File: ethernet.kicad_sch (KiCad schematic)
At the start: 22 parts, among them J2 L834-1G1T-S7, Q2 PMOS_Substrate, U2 LAN8830T_PSA

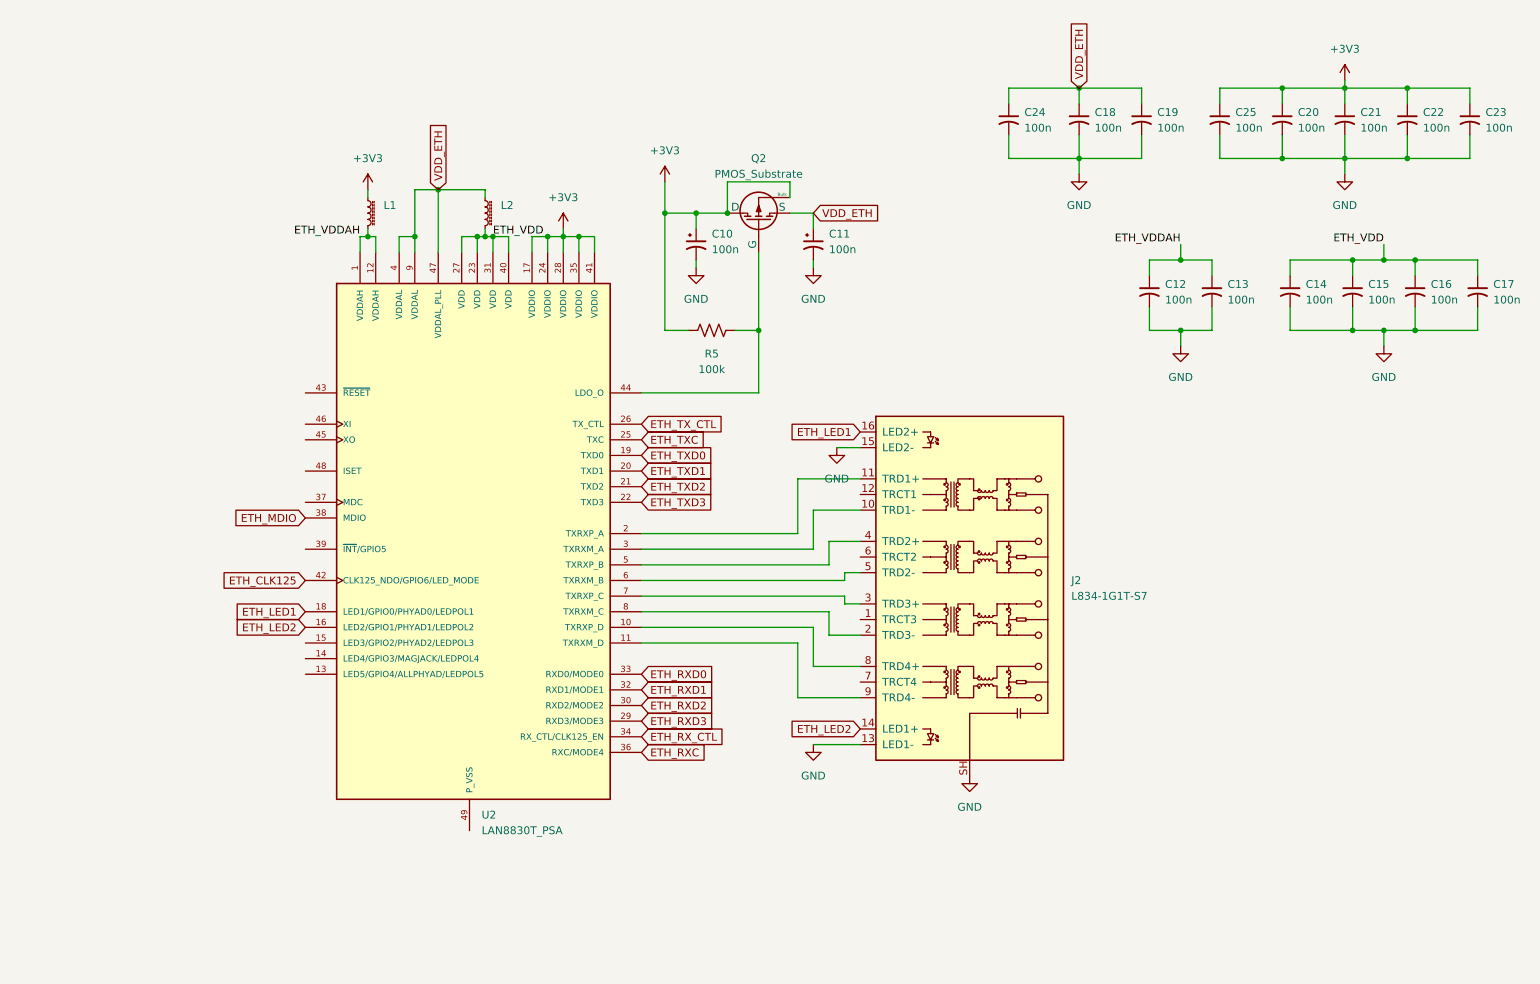
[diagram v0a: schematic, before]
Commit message: Start of ethernet
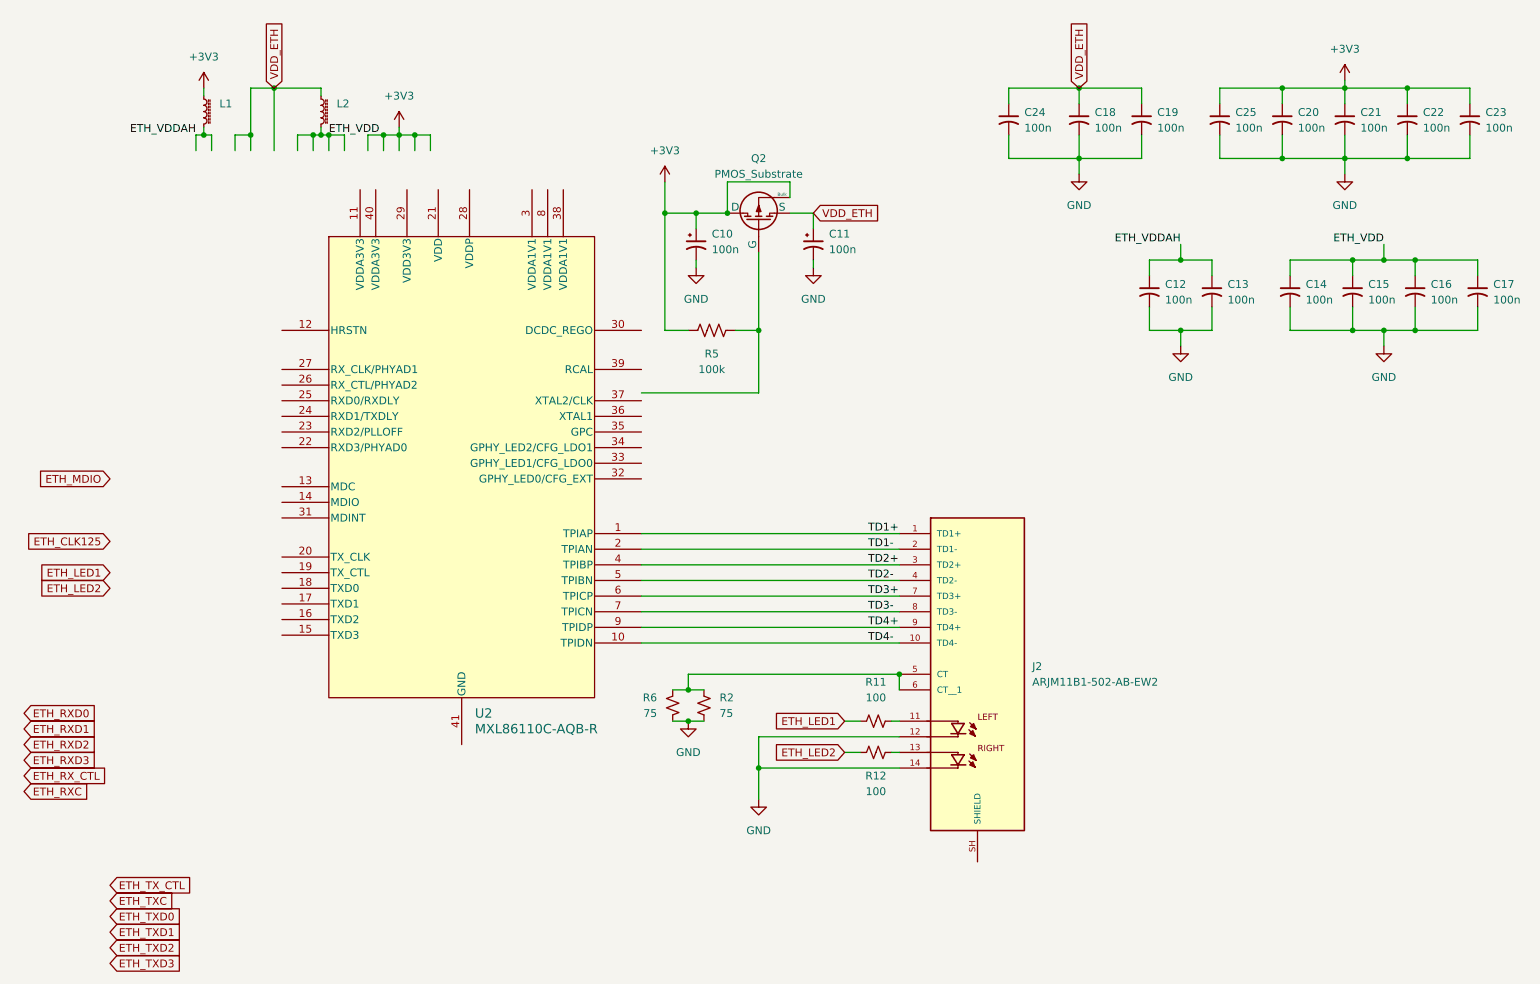
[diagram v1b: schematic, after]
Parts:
- removed J2: L834-1G1T-S7, L834-1G1T-S7:BEL_L834-1G1T-S7, symbol Library:L834-1G1T-S7
- removed U2: LAN8830T_PSA, LAN8830T_PSA:QFN50P700X700X100-49N, symbol Library:LAN8830T_PSA
- added J2: ARJM11B1-502-AB-EW2, Library:ABRACON_ARJM11B1-502-AB-EW2, symbol Library:ARJM11B1-502-AB-EW2
- added R11, R12: 100, symbol Device:R_Small_US
- added R2, R6: 75, symbol Device:R_Small_US
- added U2: MXL86110C-AQB-R, QFN40_5X5_MXL, symbol Library:MXL86110C-AQB-R
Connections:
- net ETH_LED1: now also R11.2
- net ETH_LED2: now also R12.2
- net GND: now also J2.12, J2.14, R2.1, R6.1
- new net: J2.11, R11.1
- new net: J2.13, R12.1
- new net: J2.5 (CT), J2.6 (CT__1), R2.2, R6.2
- new net TD1+: J2.1 (TD1+), U2.1 (TPIAP)
- new net TD1-: J2.2 (TD1-), U2.2 (TPIAN)
- new net TD2+: J2.3 (TD2+), U2.4 (TPIBP)
- new net TD2-: J2.4 (TD2-), U2.5 (TPIBN)
- new net TD3+: J2.7 (TD3+), U2.6 (TPICP)
- new net TD3-: J2.8 (TD3-), U2.7 (TPICN)
- new net TD4+: J2.9 (TD4+), U2.9 (TPIDP)
- new net TD4-: J2.10 (TD4-), U2.10 (TPIDN)
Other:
- moved on the sheet: L1, L2
